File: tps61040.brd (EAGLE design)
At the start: 12 x 17.3 mm, 10 parts, among them U1 TPS61040DBVR

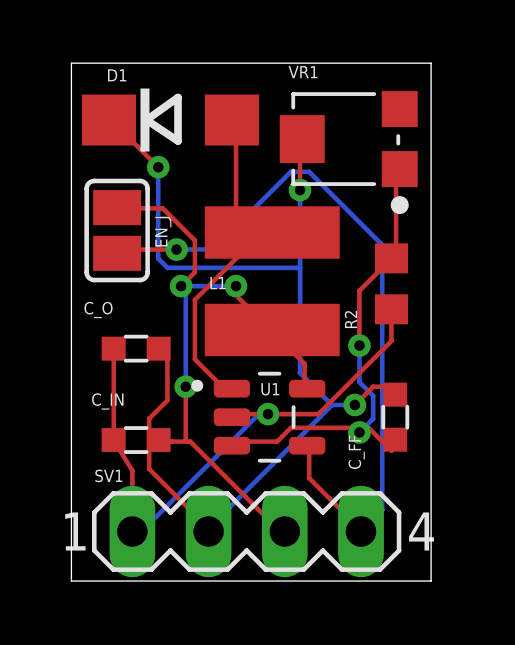
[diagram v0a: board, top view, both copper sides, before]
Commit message: update board to v1.1
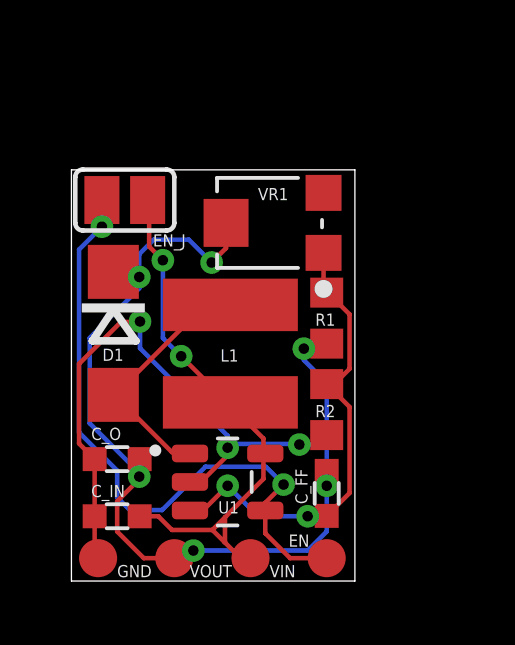
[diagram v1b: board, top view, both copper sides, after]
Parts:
- removed SV1: (no value), con-lstb:MA04-1
- added EN, GND, VIN, VOUT: TPB1,27, testpad:B1,27
- added R1: Xk, rcl:R0603
- moved D1 7.36 mm to (1.40, 8.26), turned to 270 degrees
- moved R2 4.71 mm to (8.51, 5.71)
- moved VR1 3.78 mm to (6.60, 11.9)
- moved C_O 3.74 mm to (1.52, 4.06)
- moved C_FF 3.42 mm to (8.51, 2.92)
- moved L1 2.79 mm to (3.05, 5.08)
- moved C_IN 2.62 mm to (1.52, 2.16)
- moved U1 2.57 mm to (5.21, 3.30)
- moved EN_J 1.05 mm to (1.78, 12.7), turned to 180 degrees
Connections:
- net EN: now also EN.TP; no longer SV1.4
- net GND: now also GND.TP; no longer SV1.1
- net N$2: now also R1.1
- net VIN: now also VIN.TP; no longer SV1.3
- net VOUT: now also R1.2, VOUT.TP; no longer SV1.2
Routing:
- net N$1: track 11.9 -> 8.47 mm
- net VIN: track 21.7 -> 18.5 mm, vias 3 -> 2
- net VOUT: track 35.4 -> 32.3 mm, vias 3 -> 6
- net EN: track 24.5 -> 21.6 mm, vias 1 -> 2
- net N$2: track 16.1 -> 15.6 mm
- net GND: track 19.8 -> 20.2 mm, vias 1 -> 3
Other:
- board size 12 x 17.3 mm -> 9.4 x 13.7 mm
- board text added: "TPS61040 v1.1 By DoganM95"

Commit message: update to v1.2
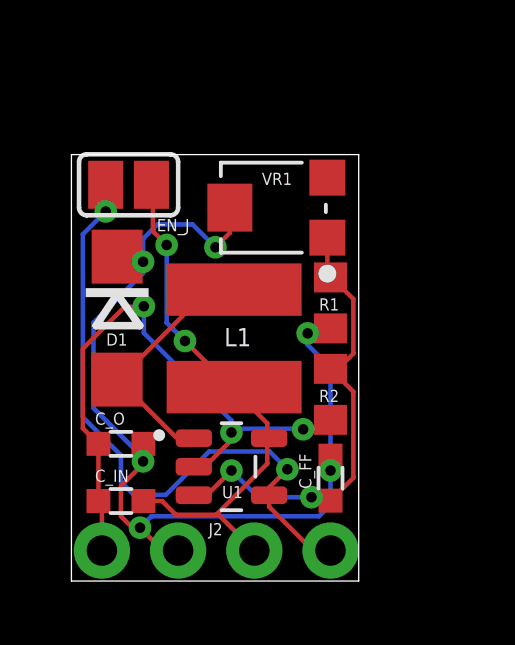
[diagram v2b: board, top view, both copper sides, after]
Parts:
- removed EN, GND, VIN, VOUT: TPB1,27, testpad:B1,27
- added J2: (no value), SparkFun-Connectors:1X04_NO_SILK
- D1: value SS54 -> SS14
- R1: value Xk -> xxxk
- R2: value 1k -> 100k
- U1: value TPS61040DBVR -> TPS61040
- VR1: value 10k -> 1M
- moved EN_J 0.52 mm to (1.91, 13.2)
- moved R1 0.52 mm to (8.64, 9.27)
- moved C_IN 0.52 mm to (1.65, 2.67)
- moved C_O 0.52 mm to (1.65, 4.57)
- moved L1 0.52 mm to (3.17, 5.59)
- moved U1 0.52 mm to (5.33, 3.81)
- moved C_FF 0.52 mm to (8.64, 3.43)
- moved R2 0.52 mm to (8.64, 6.22)
- moved D1 0.52 mm to (1.52, 8.76)
- moved VR1 0.52 mm to (6.73, 12.4)
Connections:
- net EN: now also J2.4; no longer EN.TP
- net GND: now also J2.1; no longer GND.TP
- net VIN: now also J2.3; no longer VIN.TP
- net VOUT: now also J2.2; no longer VOUT.TP
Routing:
- net VOUT: track 32.3 -> 33.3 mm
- net VIN: track 18.5 -> 17.8 mm
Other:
- board size 9.4 x 13.7 mm -> 9.6 x 14.2 mm
- board text added: "EN"
- board text added: "GND"
- board text added: "TPS61040 v1.2 By DoganM95"
- board text added: "VIN"
- board text added: "VOUT"
- board text removed: "TPS61040 v1.1 By DoganM95"
